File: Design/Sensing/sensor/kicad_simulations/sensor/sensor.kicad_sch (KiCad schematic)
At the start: 38 parts, among them J1 Conn_01x02_Pin, J10 Conn_01x02_Pin, J11 Conn_01x02_Pin, J12 Conn_01x02_Pin, J13 Conn_01x02_Pin, J14 Conn_01x01_Pin, J15 Conn_01x01_Pin, J16 Conn_01x02_Pin, J17 Conn_01x02_Pin, J2 Conn_01x02_Pin, J3 Conn_02x14_Odd_Even, J5 L_S_B, J6 Conn_01x01_Pin, J7 Conn_01x02_Pin, J8 Conn_01x02_Pin, J9 Conn_01x02_Pin, Q1 MMBT5551L, Q2 MMBT5551L, Q3 MMBT5551L, U1 LM324, U2 TSSP58038, U3 TSSP58038, U4 TSSP58038

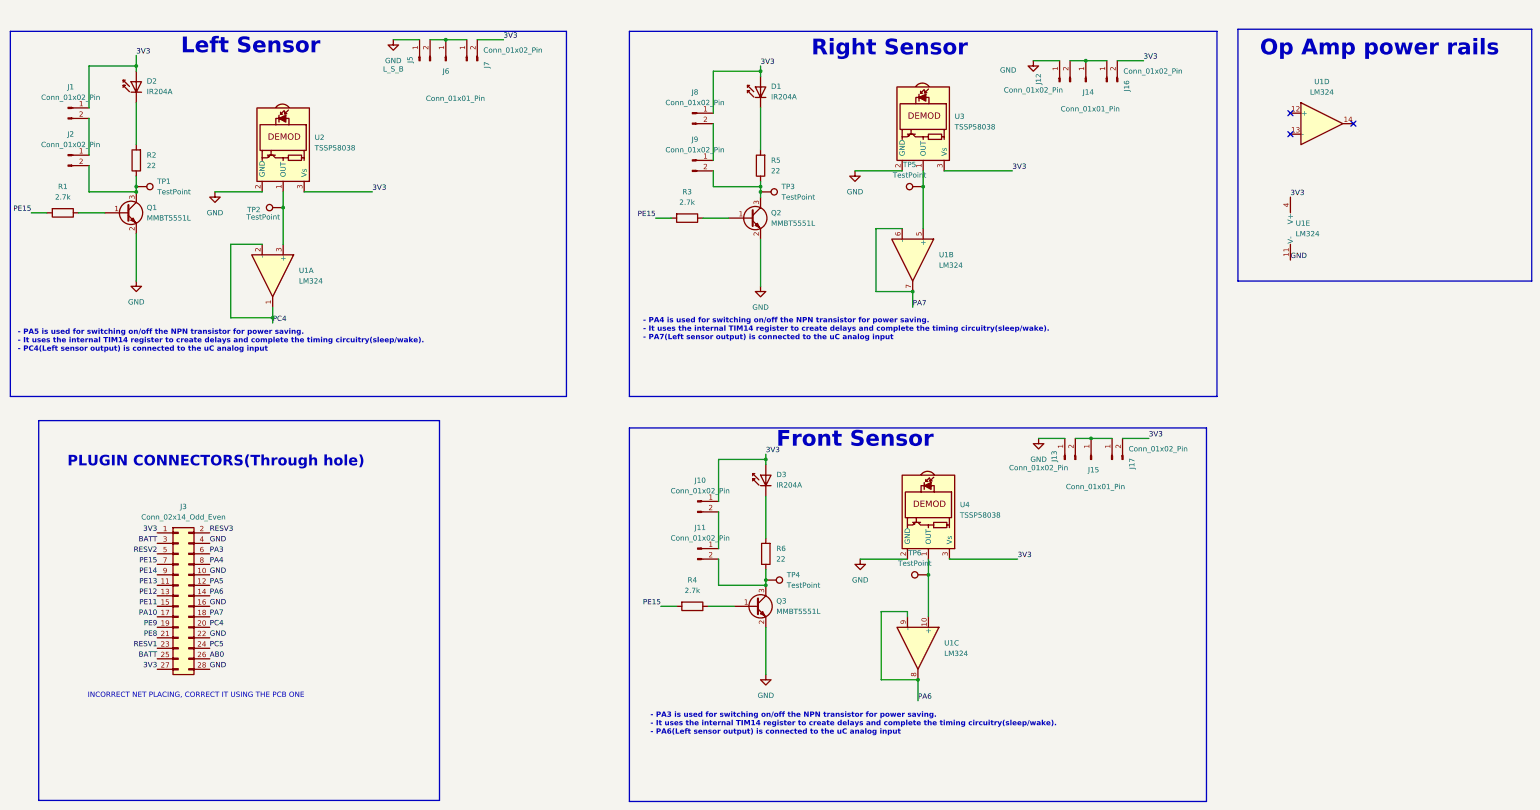
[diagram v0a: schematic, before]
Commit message: Updated the schematic
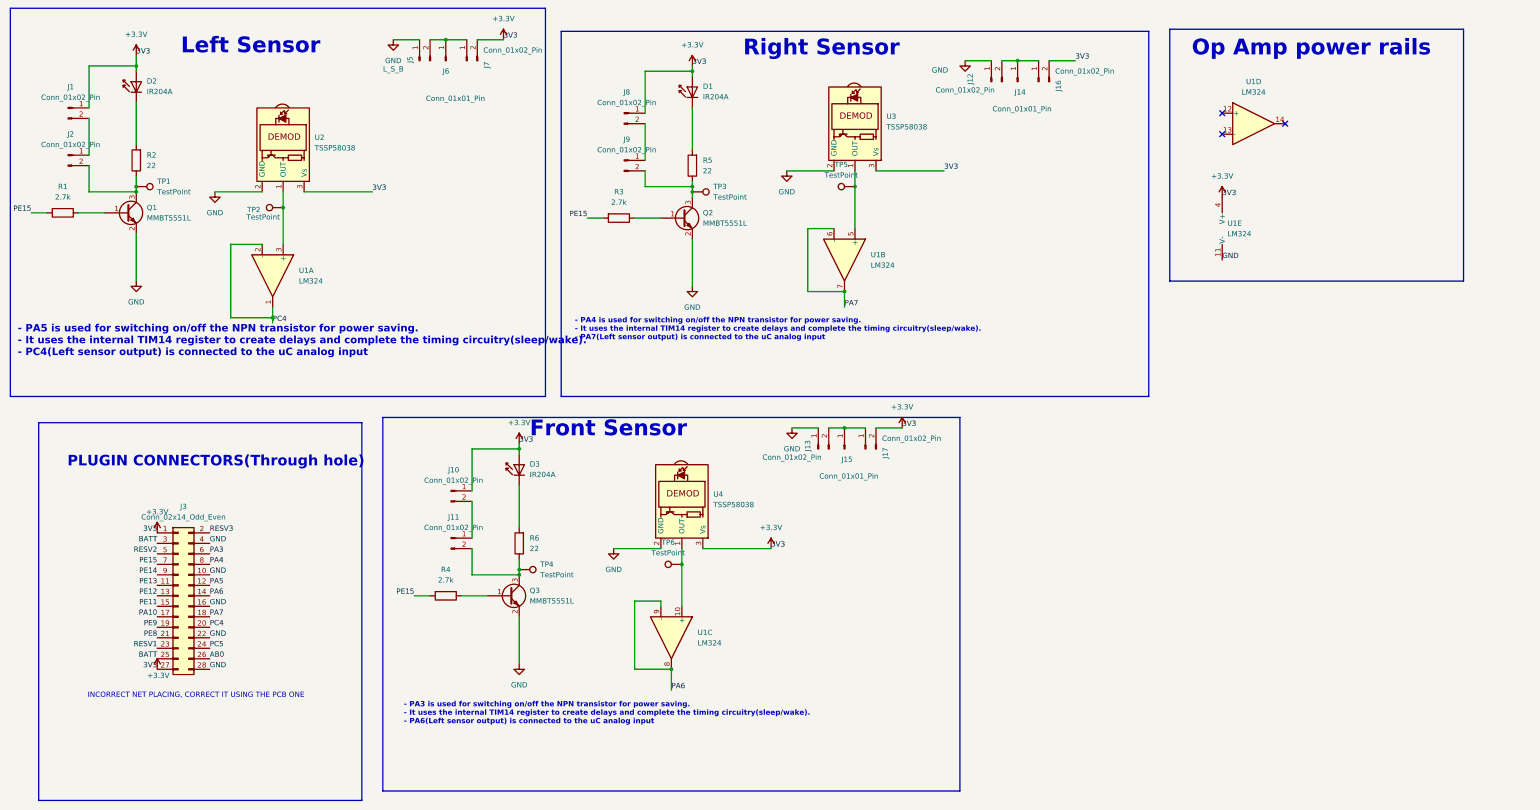
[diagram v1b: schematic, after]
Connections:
- net 3V3 renamed +3.3V
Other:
- company: (none) -> University of Cape Town
- moved on the sheet: D1, D3, J10, J11, J12, J13, J14, J15, J16, J17, J8, J9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
